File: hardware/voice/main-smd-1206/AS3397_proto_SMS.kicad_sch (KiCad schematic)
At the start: 105 parts, among them J1 ES, Q1 BS170F, Q2 BS170F, Q3 BS170F, Q4 BS170F, Q5 BS170F, U1 TS922, U2 Pico, U3 TS922, U4 TL072, U5 TS922, U6 74HC4050, U7 TS922

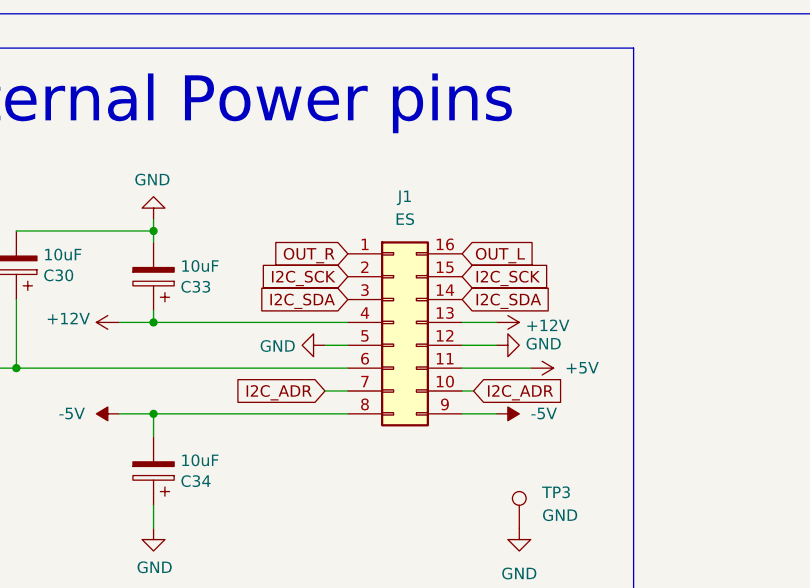
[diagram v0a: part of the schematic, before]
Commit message: Modif of voice board smd and Cleanup
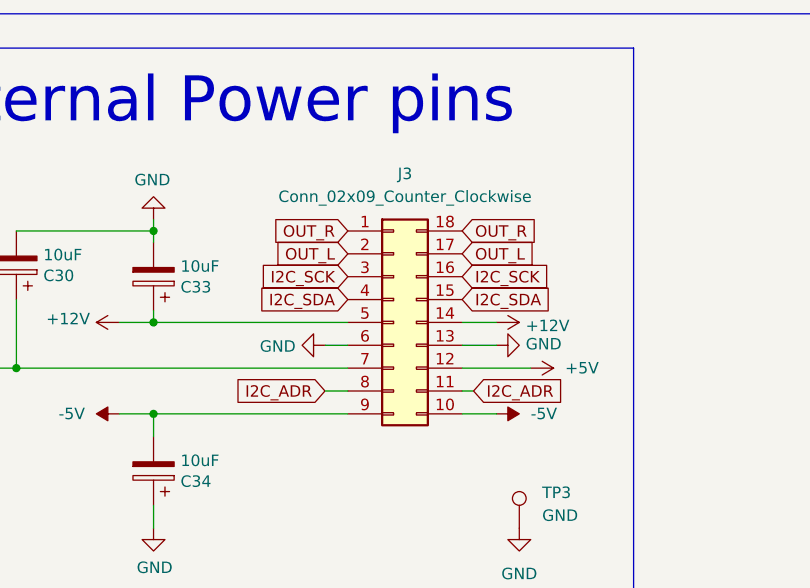
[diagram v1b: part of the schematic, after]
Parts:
- removed J1: ES, SYNTHFILLE:DIP-16_AS, symbol Connector_Generic:Conn_02x08_Counter_Clockwise
- added J3: Conn_02x09_Counter_Clockwise, AS3397_proto_SMS:DIP-18_AS, symbol Connector_Generic:Conn_02x09_Counter_Clockwise
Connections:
- net +12V: now also J3.14 (Pin_14), J3.5 (Pin_5)
- net +5V: now also J3.12 (Pin_12), J3.7 (Pin_7)
- net -5V: now also J3.10 (Pin_10), J3.9 (Pin_9)
- net GND: now also J3.13 (Pin_13), J3.6 (Pin_6)
- net I2C_ADR: now also J3.11 (Pin_11), J3.8 (Pin_8)
- net I2C_SCK: now also J3.16 (Pin_16), J3.3 (Pin_3)
- net I2C_SDA: now also J3.15 (Pin_15), J3.4 (Pin_4)
- net OUT_L: now also J3.17 (Pin_17), J3.2 (Pin_2)
- net OUT_R: now also J3.1 (Pin_1), J3.18 (Pin_18)
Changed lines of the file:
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@@
 		)
 	)
+	(global_label "OUT_L"
+		(shape input)
+		(at 67.31 359.41 180)
+		(fields_autoplaced yes)
+		(effects
+			(font
+				(size 1.27 1.27)
+			)
+			(justify right)
+		)
+		(property "Intersheetrefs" "${INTERSHEET_REFS}"
+			(at 58.7005 359.41 0)
+			(effects
+				(font
+					(size 1.27 1.27)
+				)
+				(justify right)
+				(hide yes)
+			)
+		)
+	)
 	(global_label "PWM_3.3V_PAN_CV"
 		(shape input)
@@
 		)
 	)
-	(global_label "OUT_R"
-		(shape input)
-		(at 67.31 359.41 180)
-		(fields_autoplaced yes)
-		(effects
-			(font
-				(size 1.27 1.27)
-			)
-			(justify right)
-		)
-		(property "Intersheetrefs" "${INTERSHEET_REFS}"
-			(at 58.538 359.41 0)
-			(effects
-				(font
-					(size 1.27 1.27)
-				)
-				(justify right)
-				(hide yes)
-			)
-		)
-	)
 	(global_label "PWM_5V_LINEAR_GAIN_CV"
 		(shape input)
@@
 		)
 	)
+	(global_label "OUT_R"
+		(shape input)
+		(at 80.01 356.87 0)
+		(fields_autoplaced yes)
+		(effects
+			(font
+				(size 1.27 1.27)
+			)
+			(justify left)
+		)
+		(property "Intersheetrefs" "${INTERSHEET_REFS}"
+			(at 88.8614 356.87 0)
+			(effects
+				(font
+					(size 1.27 1.27)
+				)
+				(justify left)
+				(hide yes)
+			)
+		)
+	)
 	(global_label "OUT_L"
 		(shape input)
@@
 		)
 	)
+	(global_label "OUT_R"
+		(shape input)
+		(at 67.31 356.87 180)
+		(fields_autoplaced yes)
+		(effects
+			(font
+				(size 1.27 1.27)
+			)
+			(justify right)
+		)
+		(property "Intersheetrefs" "${INTERSHEET_REFS}"
+			(at 58.538 356.87 0)
+			(effects
+				(font
+					(size 1.27 1.27)
+				)
+				(justify right)
+				(hide yes)
+			)
+		)
+	)
 	(global_label "PWM_5V_FITLER_FREQ_CV"
 		(shape output)
@@
 	)
 	(symbol
-		(lib_id "Connector_Generic:Conn_02x08_Counter_Clockwise")
-		(at 72.39 367.03 0)
-		(unit 1)
-		(exclude_from_sim no)
-		(in_bom yes)
-		(on_board yes)
-		(dnp no)
-		(fields_autoplaced yes)
-		(property "Reference" "J1"
-			(at 73.66 353.06 0)
-			(effects
-				(font
-					(size 1.27 1.27)
-				)
-			)
-		)
-		(property "Value" "ES"
-			(at 73.66 355.6 0)
-			(effects
-				(font
-					(size 1.27 1.27)
-				)
-			)
-		)
-		(property "Footprint" "SYNTHFILLE:DIP-16_AS"
-			(at 72.39 367.03 0)
-			(effects
-				(font
-					(size 1.27 1.27)
-				)
-				(hide yes)
-			)
-		)
-		(property "Datasheet" "~"
-			(at 72.39 367.03 0)
-			(effects
-				(font
-					(size 1.27 1.27)
-				)
-				(hide yes)
-			)
-		)
-		(property "Description" ""
-			(at 72.39 367.03 0)
-			(effects
-				(font
-					(size 1.27 1.27)
-				)
-			)
-		)
-		(pin "1"
-		)
-		(pin "10"
-		)
-		(pin "11"
-		)
-		(pin "12"
-		)
-		(pin "13"
-		)
-		(pin "14"
-		)
-		(pin "15"
-		)
-		(pin "16"
-		)
-		(pin "2"
-		)
-		(pin "3"
-		)
-		(pin "4"
-		)
-		(pin "5"
-		)
-		(pin "6"
-		)
-		(pin "7"
-		)
-		(pin "8"
-		)
-		(pin "9"
-		)
-		(instances
-			(project "AS3397_proto_SMS"
-				(path "/43297676-3545-49e4-a57f-bd05dddc7f2c"
-					(reference "J1")
-					(unit 1)
-				)
-			)
-		)
-	)
-	(symbol
 		(lib_id "Device:R")
 		(at 227.33 231.14 0)
@@
 					(unit 1)
 				)
+			)
+		)
+	)
+	(symbol
+		(lib_id "Connector_Generic:Conn_02x09_Counter_Clockwise")
+		(at 72.39 367.03 0)
+		(unit 1)
+		(exclude_from_sim no)
+		(in_bom yes)
+		(on_board yes)
+		(dnp no)
+		(fields_autoplaced yes)
+		(property "Reference" "J3"
+			(at 73.66 350.52 0)
+			(effects
+				(font
+					(size 1.27 1.27)
+				)
+			)
+		)
+		(property "Value" "Conn_02x09_Counter_Clockwise"
+			(at 73.66 353.06 0)
+			(effects
+				(font
+					(size 1.27 1.27)
+				)
+			)
+		)
+		(property "Footprint" "AS3397_proto_SMS:DIP-18_AS"
+			(at 72.39 367.03 0)
+			(effects
+				(font
+					(size 1.27 1.27)
+				)
+				(hide yes)
+			)
+		)
+		(property "Datasheet" "~"
+			(at 72.39 367.03 0)
+			(effects
+				(font
+					(size 1.27 1.27)
+				)
+				(hide yes)
+			)
+		)
+		(property "Description" "Generic connector, double row, 02x09, counter clockwise pin numbering scheme (similar to DIP package numbering), script generated (kicad-library-utils/schlib/autogen/connector/)"
+			(at 72.39 367.03 0)
+			(effects
+				(font
+					(size 1.27 1.27)
+				)
+				(hide yes)
+			)
+		)
+		(pin "14"
+		)
+		(pin "18"
+		)
+		(pin "16"
+		)
+		(pin "9"
+		)
+		(pin "11"
+		)
+		(pin "5"
+		)
+		(pin "6"
+		)
+		(pin "7"
+		)
+		(pin "13"
+		)
+		(pin "15"
+		)
+		(pin "10"
+		)
+		(pin "8"
+		)
+		(pin "17"
+		)
+		(pin "1"
+		)
+		(pin "2"
+		)
+		(pin "4"
+		)
+		(pin "3"
+		)
+		(pin "12"
+		)
+		(instances
+			(project ""
+				(path "/43297676-3545-49e4-a57f-bd05dddc7f2c"
+					(reference "J3")
+					(unit 1)
+				)
